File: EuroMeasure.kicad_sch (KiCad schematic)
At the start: 33 parts, among them SW1 SW_DIP_x04, SW2 RST, U10 AZ1117-3V3, U11 STM32G030CxT, Y1 16MHz

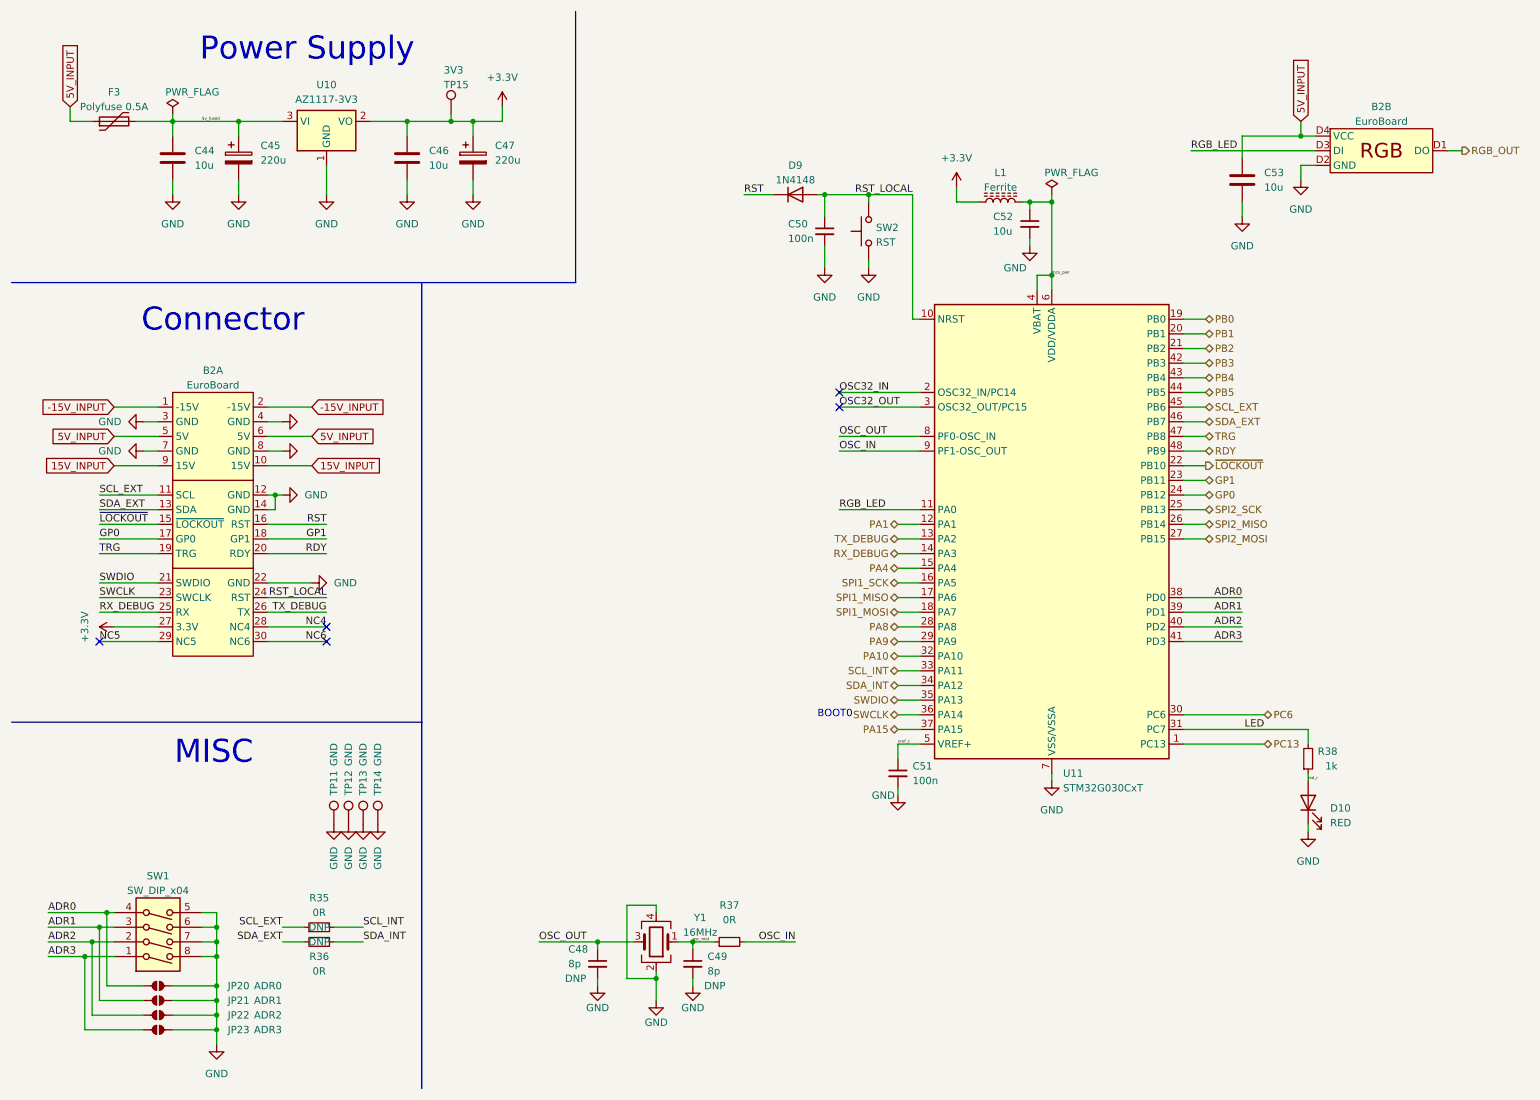
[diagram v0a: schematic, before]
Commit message: Cleaned up PCB
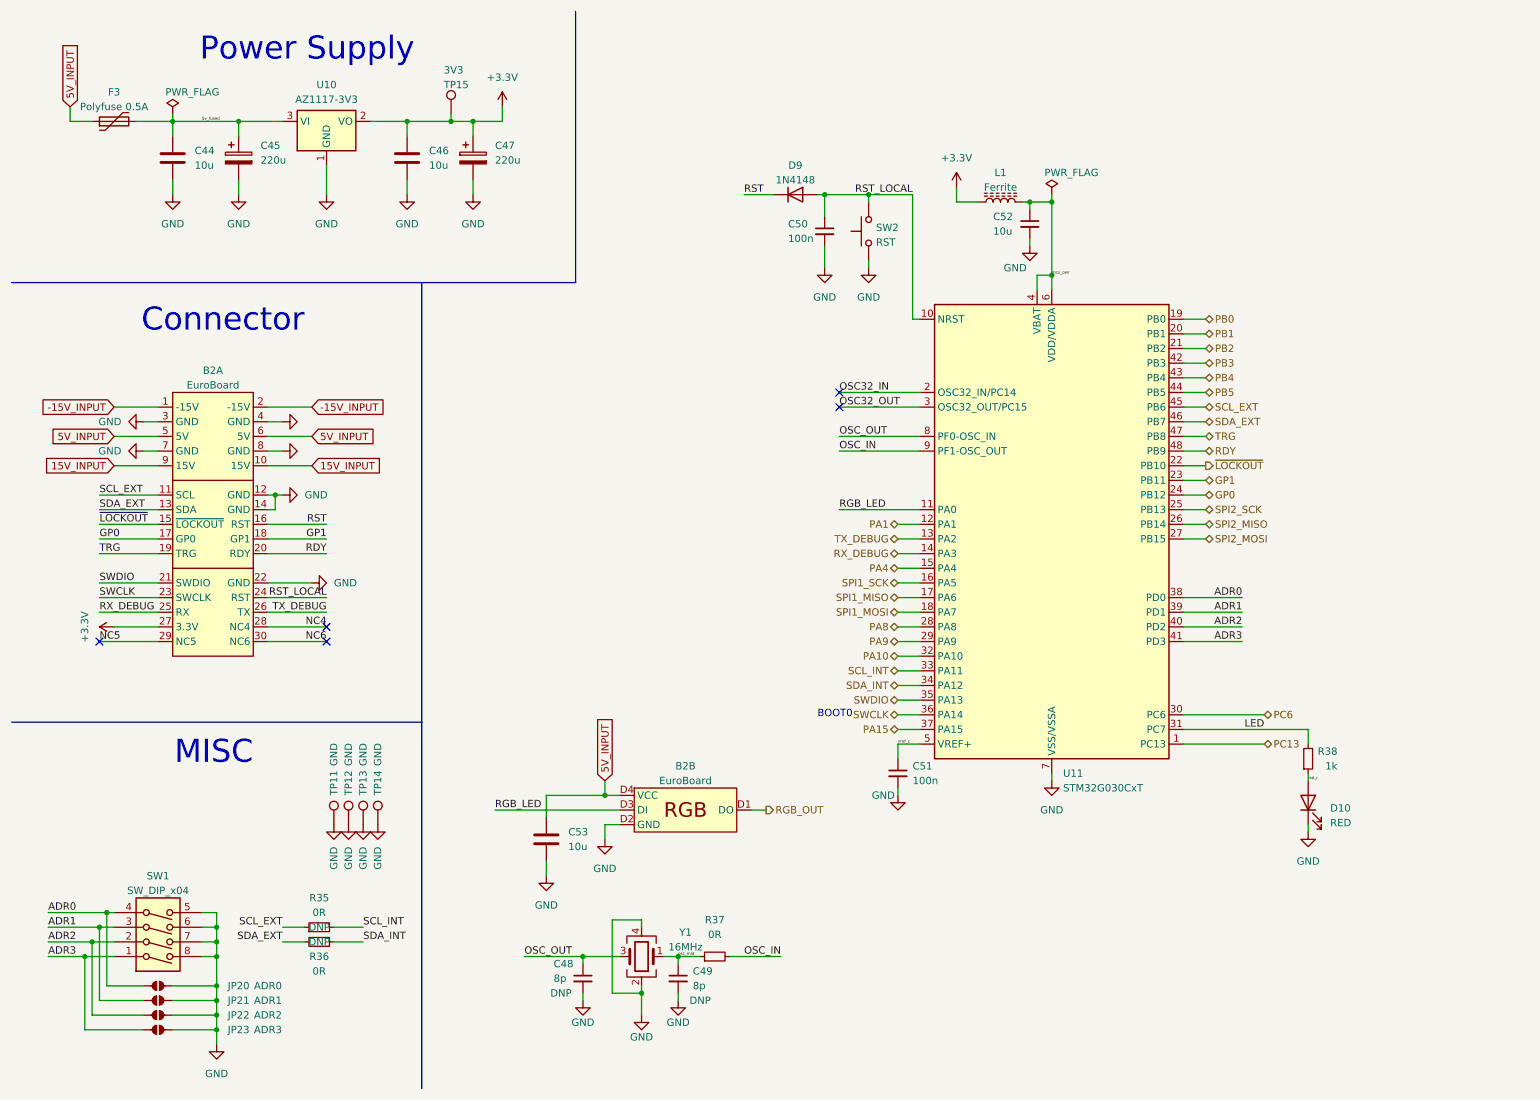
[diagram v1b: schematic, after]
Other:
- moved on the sheet: B2B, C48, C49, C53, R37, Y1
